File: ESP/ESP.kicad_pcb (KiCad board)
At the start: 4 copper layers, 33.7 x 17.8 mm, 28 parts, among them J3 USB_B_Micro, J4 Micro_SD_Card_Det, Q1 mmbt2222, Q2 mmbt2222, U1 ESP32-PICO-D4, U2 AP2112K-3.3, U3 CP2104

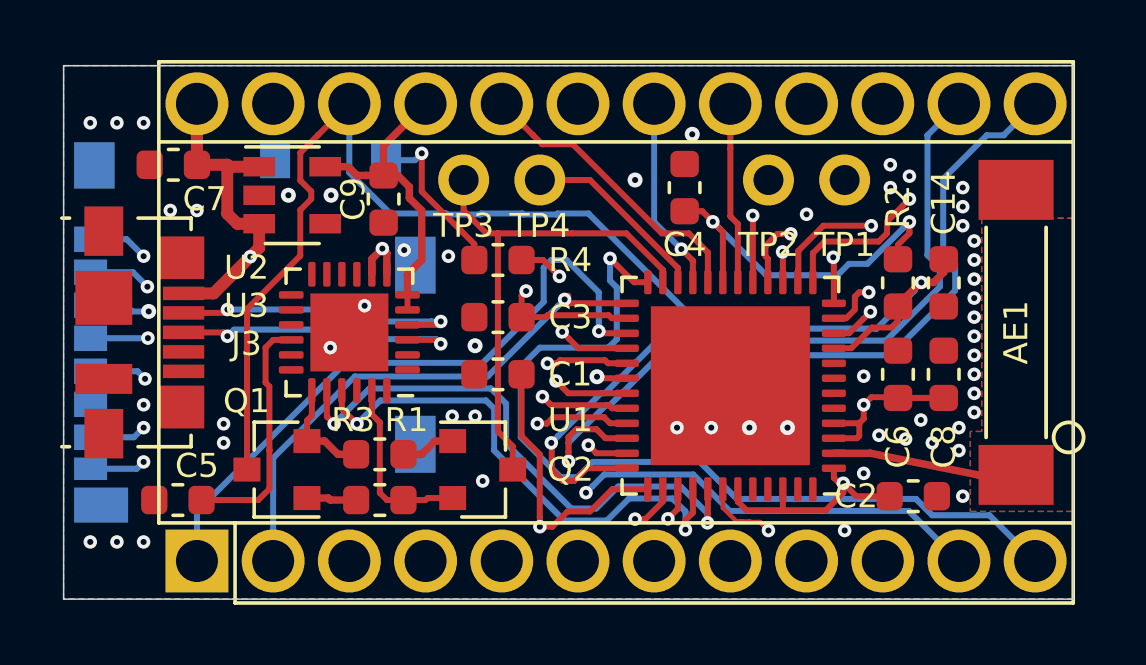
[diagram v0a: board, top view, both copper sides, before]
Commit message: blindly dumped everything
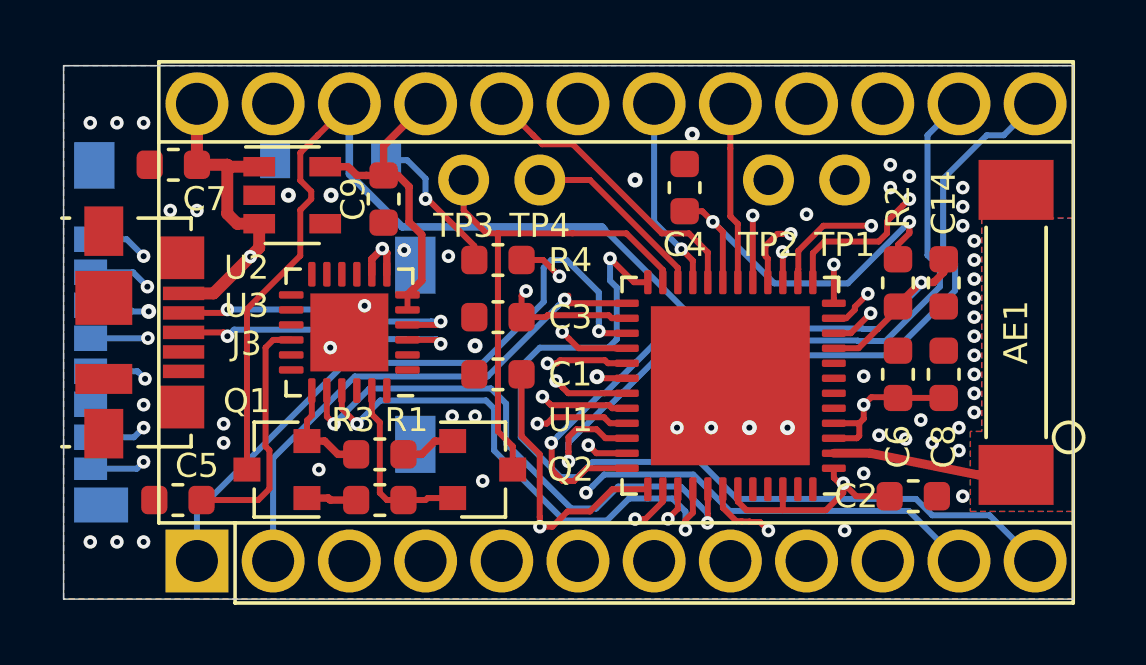
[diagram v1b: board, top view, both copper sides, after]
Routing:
- net Net-(J4-Pad10): track 5.56 -> 5.00 mm
- net GND: vias 54 -> 55
